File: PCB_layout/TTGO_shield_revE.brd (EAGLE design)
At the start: 113.1 x 113.1 mm, 30 parts

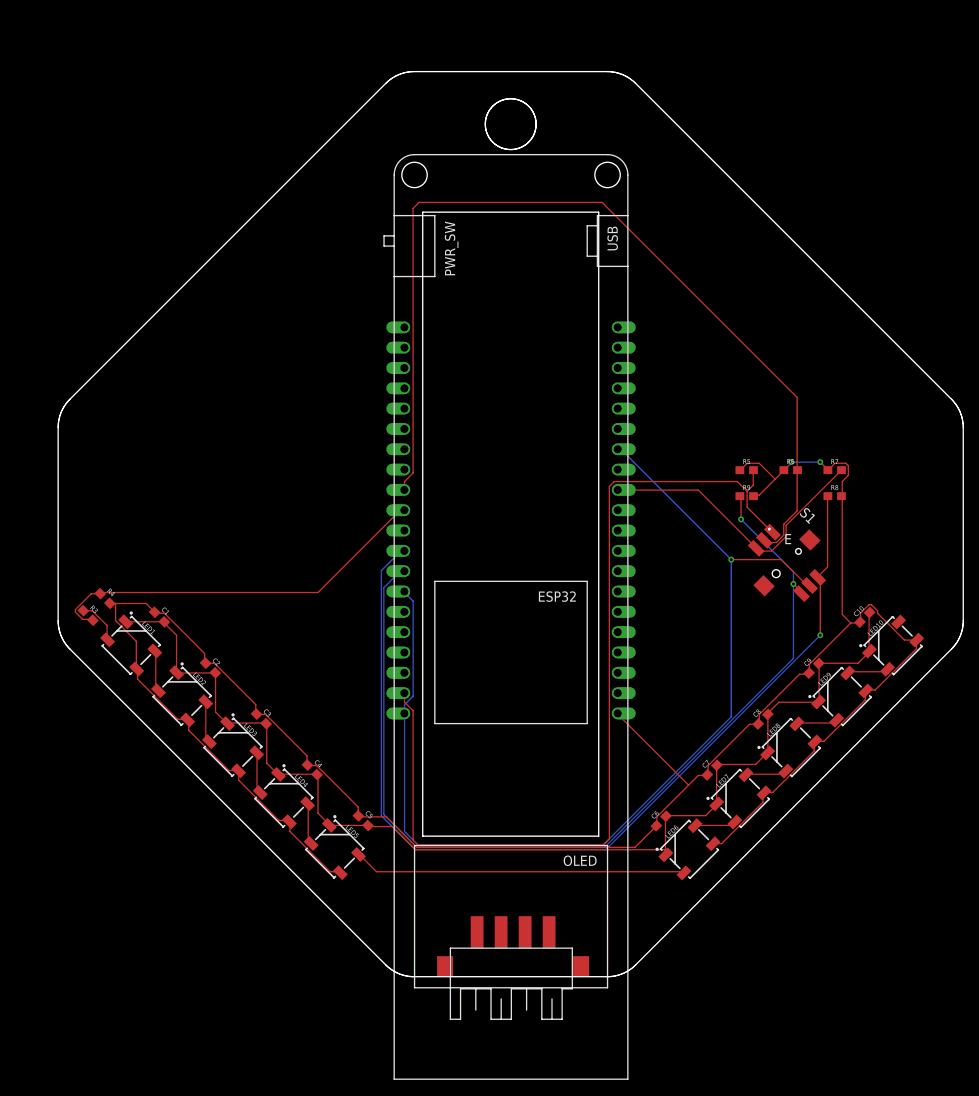
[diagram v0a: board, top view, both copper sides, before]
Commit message: RevE off to fab house!
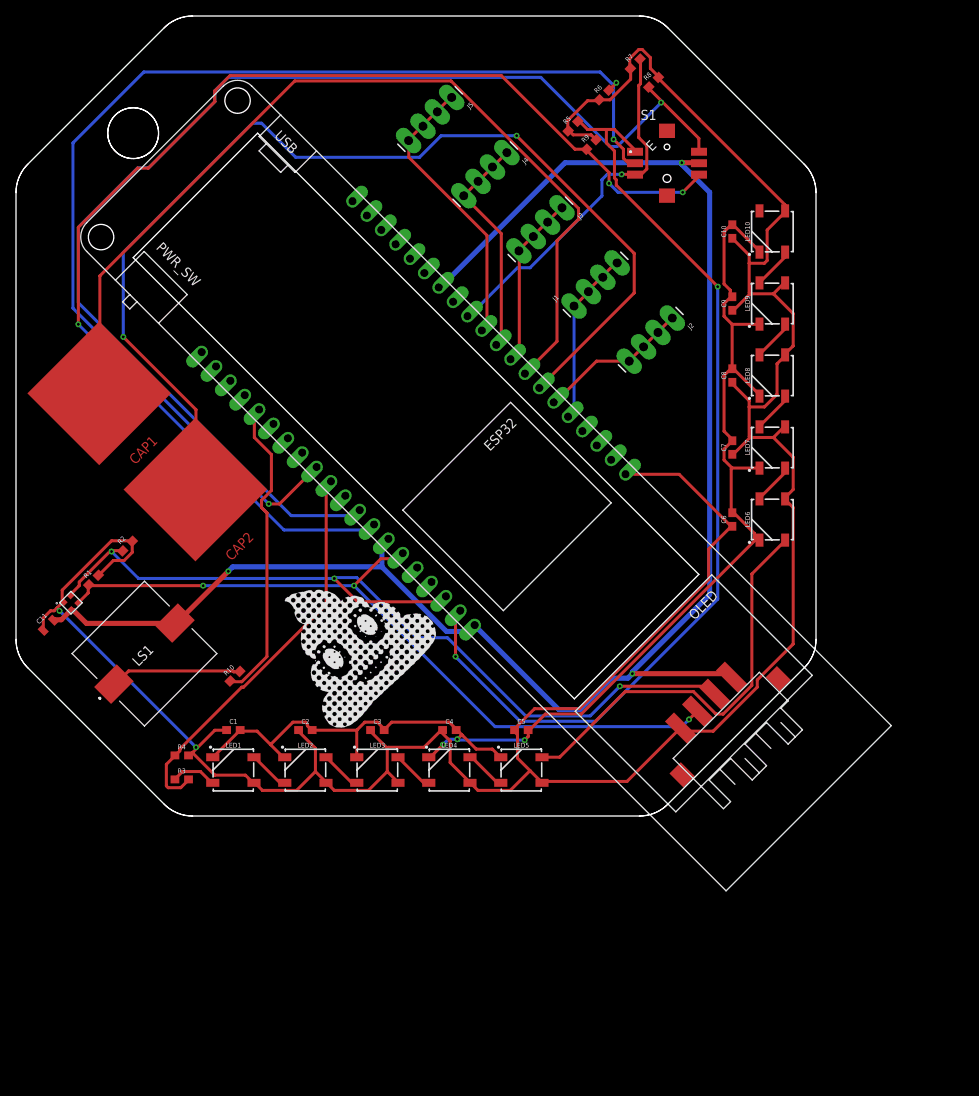
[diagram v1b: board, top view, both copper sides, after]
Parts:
- removed U$1: 10120045-400LF, BadgeParts:10120045-400LF
- added C11: 1.0uF, SparkFun-Capacitors:0805
- added CAP1, CAP2: CAPSENSE_BUTTON, BadgeParts:CAPSENSE_BUTTON
- added HEMA1: 10120045-400LF, BadgeParts:10120045-400LF
- added J1, J2, J3, J4, J5: (no value), SparkFun-Connectors:1X04_LONGPADS
- added LS1: CT-1205H-SMT-TR, BadgeParts:CT1205HSMTTR
- added LTSNS1: LTR-329ALS-01, NickParts:CHIPLED-4
- added R1, R2: 4.7k, SparkFun-Resistors:0603
- added R10: 220, SparkFun-Resistors:0603
- moved R7 56.6 mm to (65.6, 107.5), turned to 45 degrees
- moved R8 56.5 mm to (67.9, 105.2), turned to 45 degrees
- moved LED10 53.9 mm to (82.7, 86.6), turned to 90 degrees
- moved R6 52.4 mm to (61.7, 103.6), turned to 45 degrees
- moved S1 52.2 mm to (69.5, 95.1), turned to 0 degrees
- moved C10 51.0 mm to (77.7, 86.6), turned to 90 degrees
- moved LED9 49.9 mm to (82.7, 77.6), turned to 90 degrees
- moved R5 48.2 mm to (57.8, 99.8), turned to 45 degrees
- moved R9 48.1 mm to (60.1, 97.5), turned to 45 degrees
- moved C9 46.7 mm to (77.7, 77.6), turned to 90 degrees
- moved LED8 46.6 mm to (82.7, 68.6), turned to 90 degrees
- moved LED7 44.0 mm to (82.7, 59.6), turned to 90 degrees
- moved C8 43.1 mm to (77.7, 68.6), turned to 90 degrees
- moved LED6 42.5 mm to (82.7, 50.6), turned to 90 degrees
- moved C7 40.4 mm to (77.7, 59.6), turned to 90 degrees
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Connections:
- removed net CAP1: MAIN.32
- removed net CAP2: MAIN.33
- new net 15: MAIN.15, R10.1
- new net 25: J3.1, J3.2, J3.3, J3.4, MAIN.25
- new net 26: J4.1, J4.2, J4.3, J4.4, MAIN.26
- new net 27: J5.1, J5.2, J5.3, J5.4, MAIN.27
- new net 32: CAP2.1, MAIN.32
- new net 33: CAP1.1, MAIN.33
- new net 34: J1.1, J1.2, J1.3, J1.4, MAIN.34
- new net 35: J2.1, J2.2, J2.3, J2.4, MAIN.35
- new net N$7: LS1.1, R10.2
- net GND: now also C11.2, HEMA1.D, LS1.2, LTSNS1.2
- net SCL: now also HEMA1.C, LTSNS1.4, R2.1
- net SDA: now also HEMA1.B, LTSNS1.3, R1.1
- net VDD: now also C11.1, HEMA1.A, LTSNS1.1, R1.2, R2.2
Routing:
- net 32: track 0.00 -> 134.7 mm, vias 0 -> 2
- net 33: track 0.00 -> 114.7 mm
- net SCL: track 0.00 -> 110.7 mm, vias 0 -> 3
- net SDA: track 0.00 -> 94.8 mm, vias 0 -> 3
- net VDD: track 274.4 -> 362.4 mm
- net GND: track 129.8 -> 211.2 mm, vias 1 -> 3
- net 15: track 0.00 -> 38.8 mm
- net 27: track 0.00 -> 35.9 mm
- net J-LEFT: track 119.2 -> 154.1 mm, vias 2 -> 3
- net J-DOWN: track 120.3 -> 154.0 mm
- net J-PRESS: track 114.9 -> 148.2 mm, vias 0 -> 3
- net 26: track 0.00 -> 28.5 mm
- net 34: track 0.00 -> 22.1 mm
- net 25: track 0.00 -> 21.8 mm
- net GND1: track 143.7 -> 164.4 mm, vias 0 -> 3
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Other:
- board size 113.1 x 113.1 mm -> 100 x 100 mm
- board text added: "/Users/taylor/Documents/Github/CAAint/Media/Poop_Emoji_7b204f05-eec6-4496-91b1-351acc03d2c7_large.bmp"
